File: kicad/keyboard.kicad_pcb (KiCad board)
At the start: 4 copper layers, 424.4 x 124.4 mm, 183 parts, among them SW1 SW_Push, SW10 SW_Push, SW11 SW_Push, SW12 SW_Push, SW13 SW_Push, SW14 SW_Push, SW15 SW_Push, SW16 SW_Push, SW17 SW_Push, SW18 SW_Push, SW19 SW_Push, SW2 SW_Push, SW20 SW_Push, SW21 SW_Push, SW22 SW_Push, SW23 SW_Push, SW24 SW_Push, SW25 SW_Push, SW26 SW_Push, SW27 SW_Push, SW28 SW_Push, SW29 SW_Push, SW3 SW_Push, SW30 SW_Push, SW31 SW_Push, SW32 SW_Push, SW33 SW_Push, SW34 SW_Push, SW35 SW_Push, SW36 SW_Push, SW37 SW_Push, SW38 SW_Push, SW39 SW_Push, SW4 SW_Push, SW40 SW_Push, SW41 SW_Push, SW42 SW_Push, SW43 SW_Push, SW44 SW_Push, SW45 SW_Push, SW46 SW_Push, SW47 SW_Push, SW48 SW_Push, SW49 SW_Push, SW5 SW_Push, SW50 SW_Push, SW51 SW_Push, SW52 SW_Push, SW53 SW_Push, SW54 SW_Push, SW55 SW_Push, SW56 SW_Push, SW57 SW_Push, SW58 SW_Push, SW59 SW_Push, SW6 SW_Push, SW60 SW_Push, SW61 SW_Push, SW62 SW_Push, SW63 SW_Push, SW64 SW_Push, SW65 SW_Push, SW66 SW_Push, SW67 SW_Push, SW68 SW_Push, SW69 SW_Push, SW7 SW_Push, SW70 SW_Push, SW71 SW_Push, SW72 SW_Push, SW73 SW_Push, SW74 SW_Push, SW75 SW_Push, SW76 SW_Push, SW77 SW_Push, SW78 SW_Push, SW79 SW_Push, SW8 SW_Push, SW80 SW_Push, SW9 SW_Push

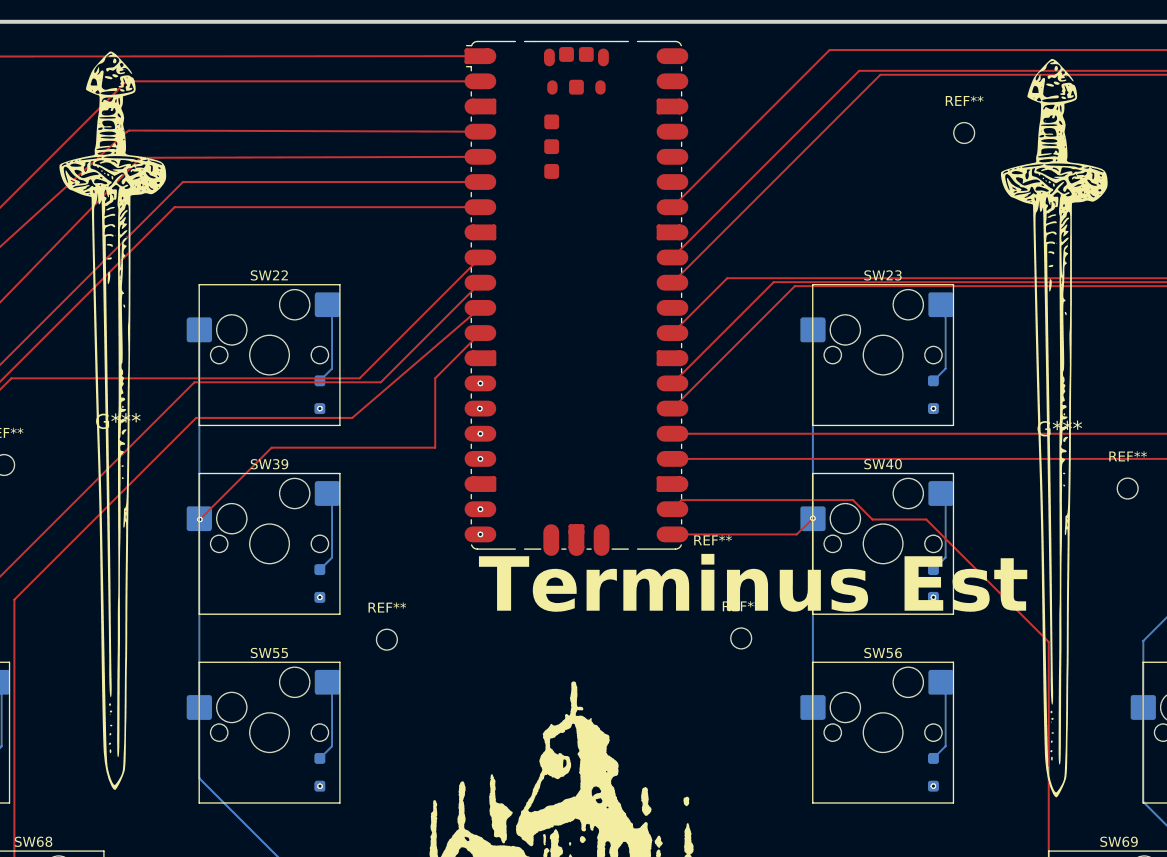
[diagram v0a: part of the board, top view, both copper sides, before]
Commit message: WIP
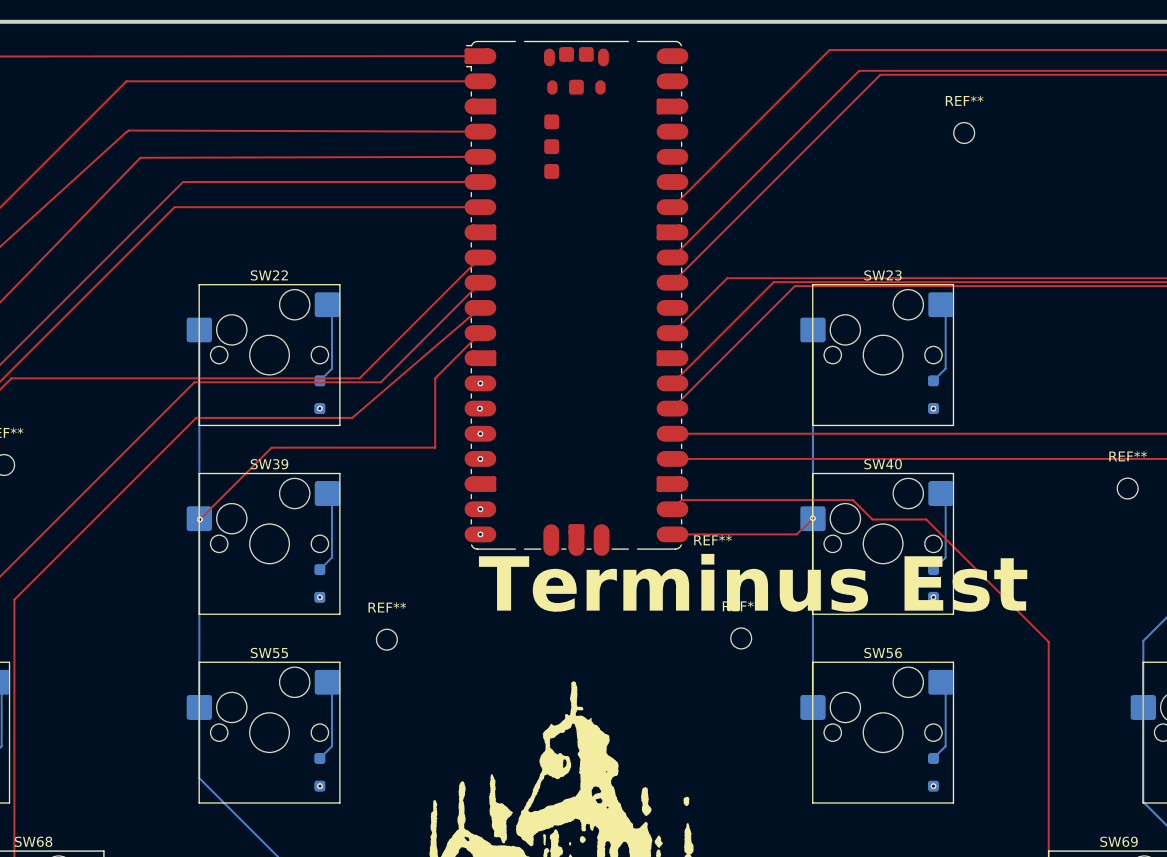
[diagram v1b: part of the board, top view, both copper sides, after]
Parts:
- removed the G*** at (249.1, 170.4)
- G***: moved to B.Cu
- moved G*** 49.2 mm to (295.7, 179.7), turned to 179 degrees
